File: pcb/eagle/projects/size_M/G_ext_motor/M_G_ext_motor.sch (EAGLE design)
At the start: 11 parts

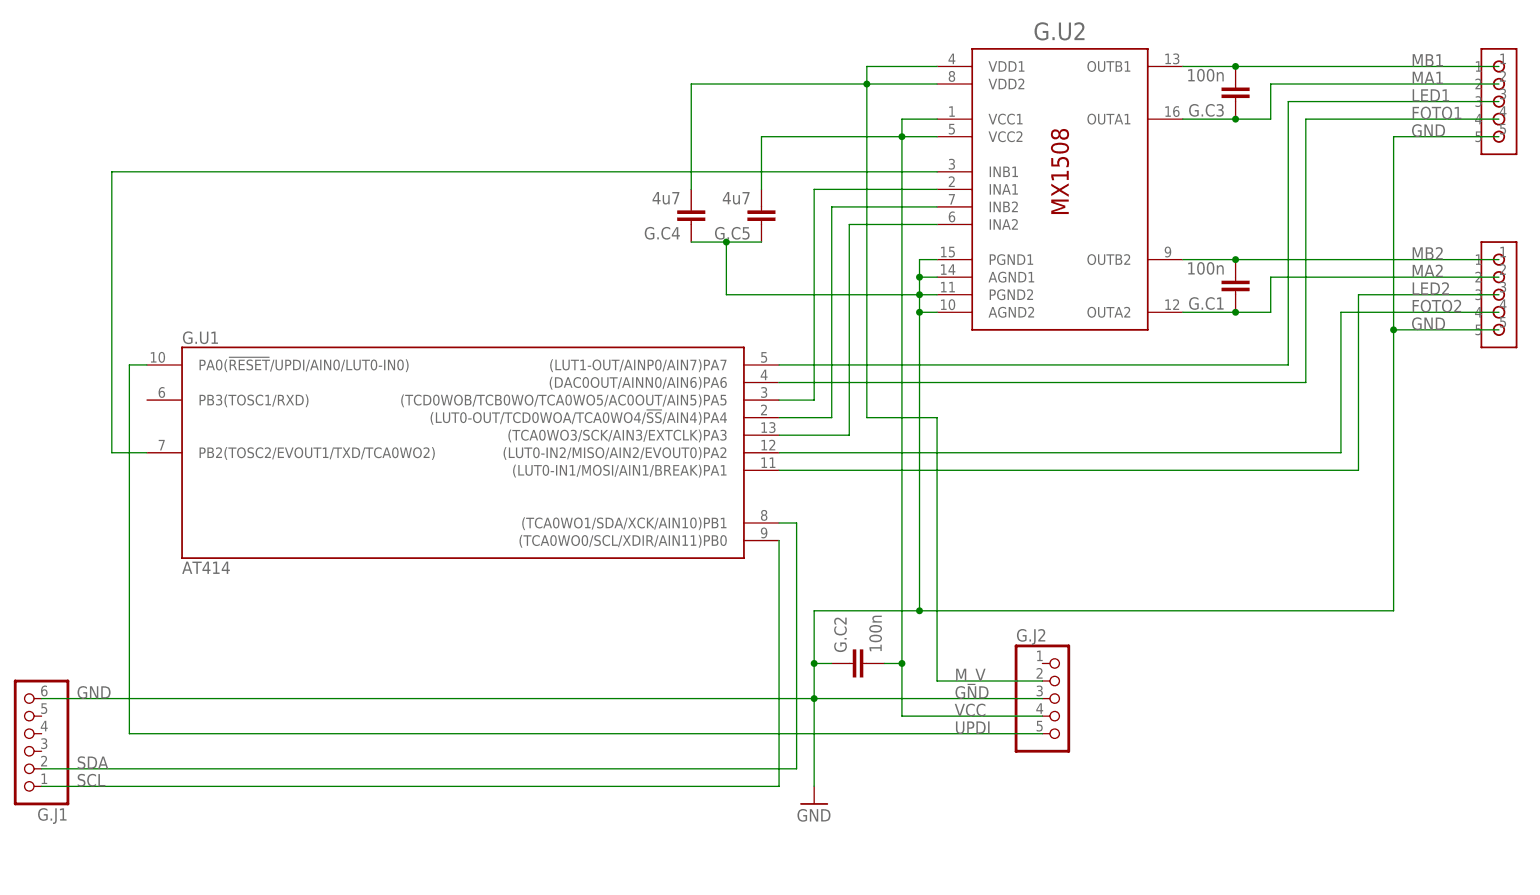
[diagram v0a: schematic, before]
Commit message: PCB M.1
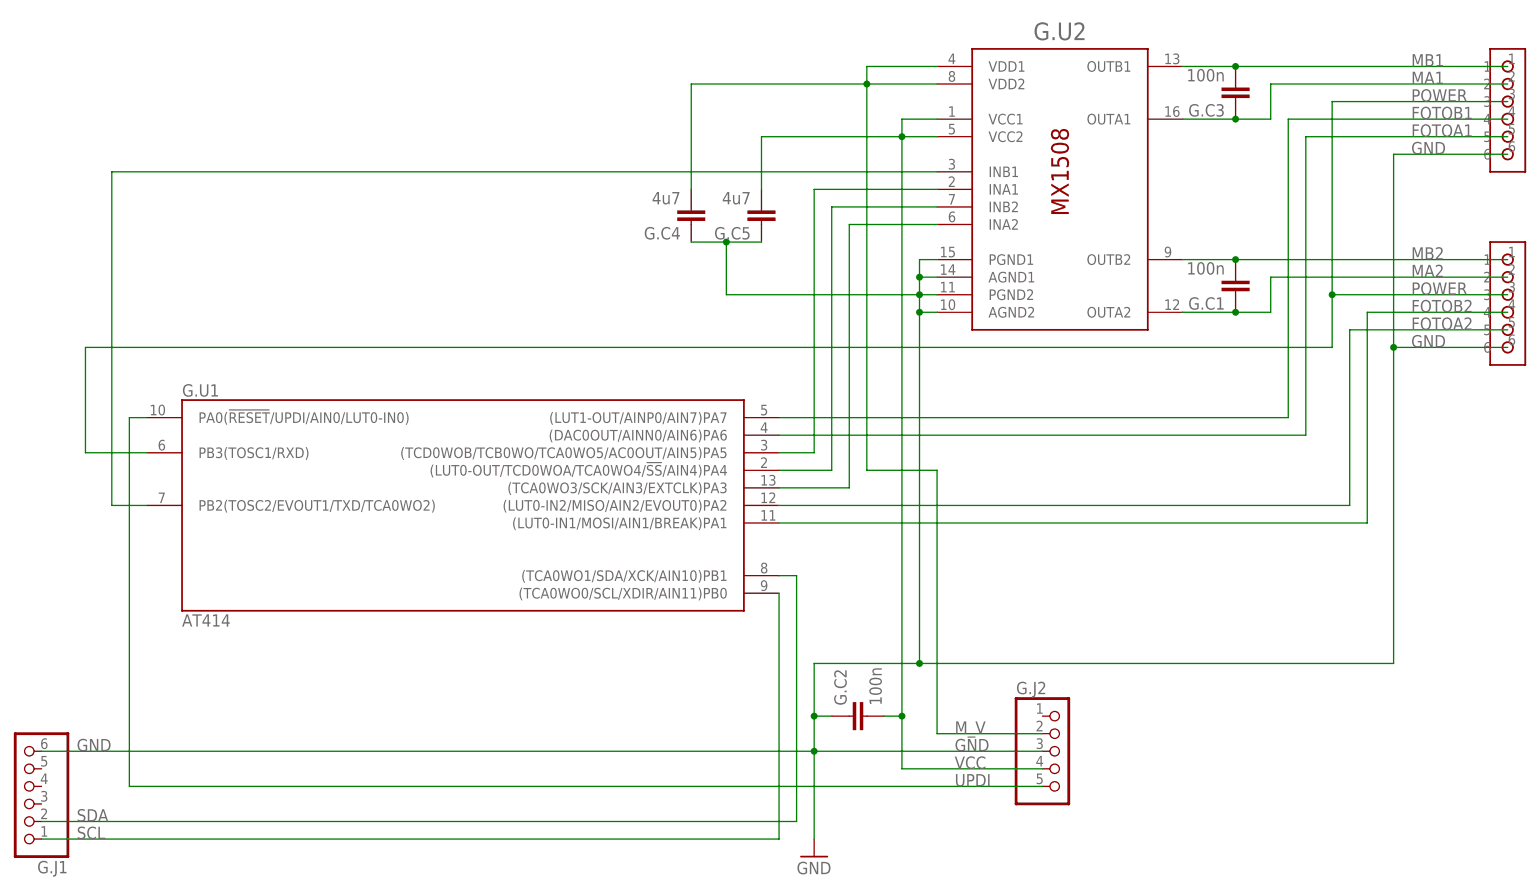
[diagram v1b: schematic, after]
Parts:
- G.J3, G.MOTO1: value A1250WR -> A1250WR-6; device hugo:A1250WR -> hugo:A1250WR-6
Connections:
- removed net FOTO1: G.MOTO1.4, G.U1G$1.(DAC0OUT/AINN0/AIN6)PA6
- removed net FOTO2: G.J3.4, G.U1G$1.(LUT0-IN2/MISO/AIN2/EVOUT0)PA2
- removed net LED1: G.MOTO1.3, G.U1G$1.(LUT1-OUT/AINP0/AIN7)PA7
- removed net LED2: G.J3.3, G.U1G$1.(LUT0-IN1/MOSI/AIN1/BREAK)PA1
- new net FOTOA1: G.MOTO1.5, G.U1G$1.(DAC0OUT/AINN0/AIN6)PA6
- new net FOTOA2: G.J3.5, G.U1G$1.(LUT0-IN2/MISO/AIN2/EVOUT0)PA2
- new net FOTOB1: G.MOTO1.4, G.U1G$1.(LUT1-OUT/AINP0/AIN7)PA7
- new net FOTOB2: G.J3.4, G.U1G$1.(LUT0-IN1/MOSI/AIN1/BREAK)PA1
- new net POWER: G.J3.3, G.MOTO1.3, G.U1G$1.PB3(TOSC1/RXD)
- net GND: now also G.J3.6, G.MOTO1.6; no longer G.J3.5, G.MOTO1.5
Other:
- moved on the sheet: G.C2, G.J1, G.J2, G.U1
